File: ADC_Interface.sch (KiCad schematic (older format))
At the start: 18 parts

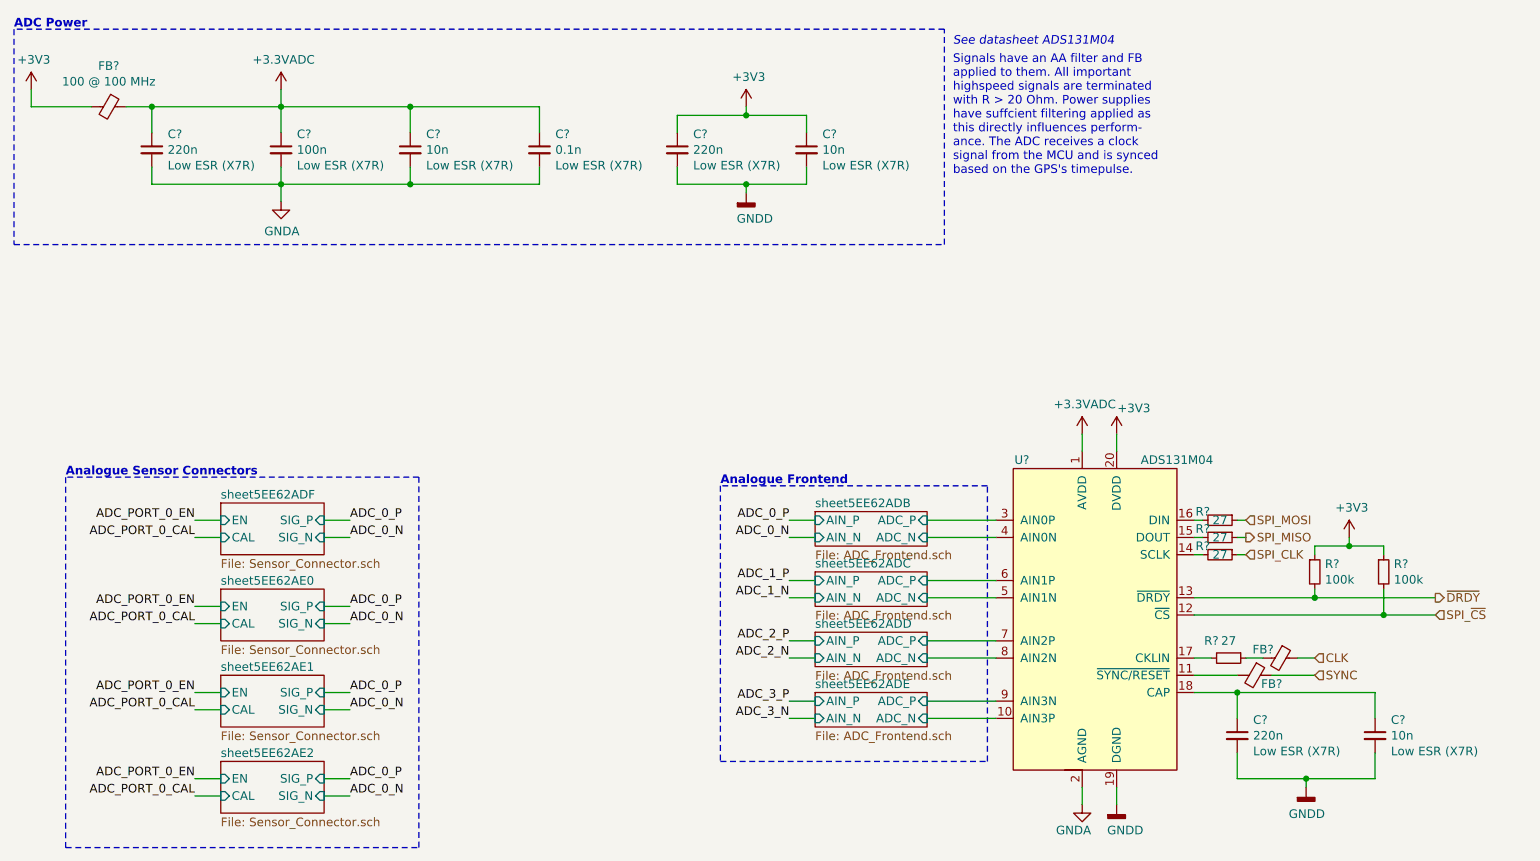
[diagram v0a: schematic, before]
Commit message: Design Mic. Board
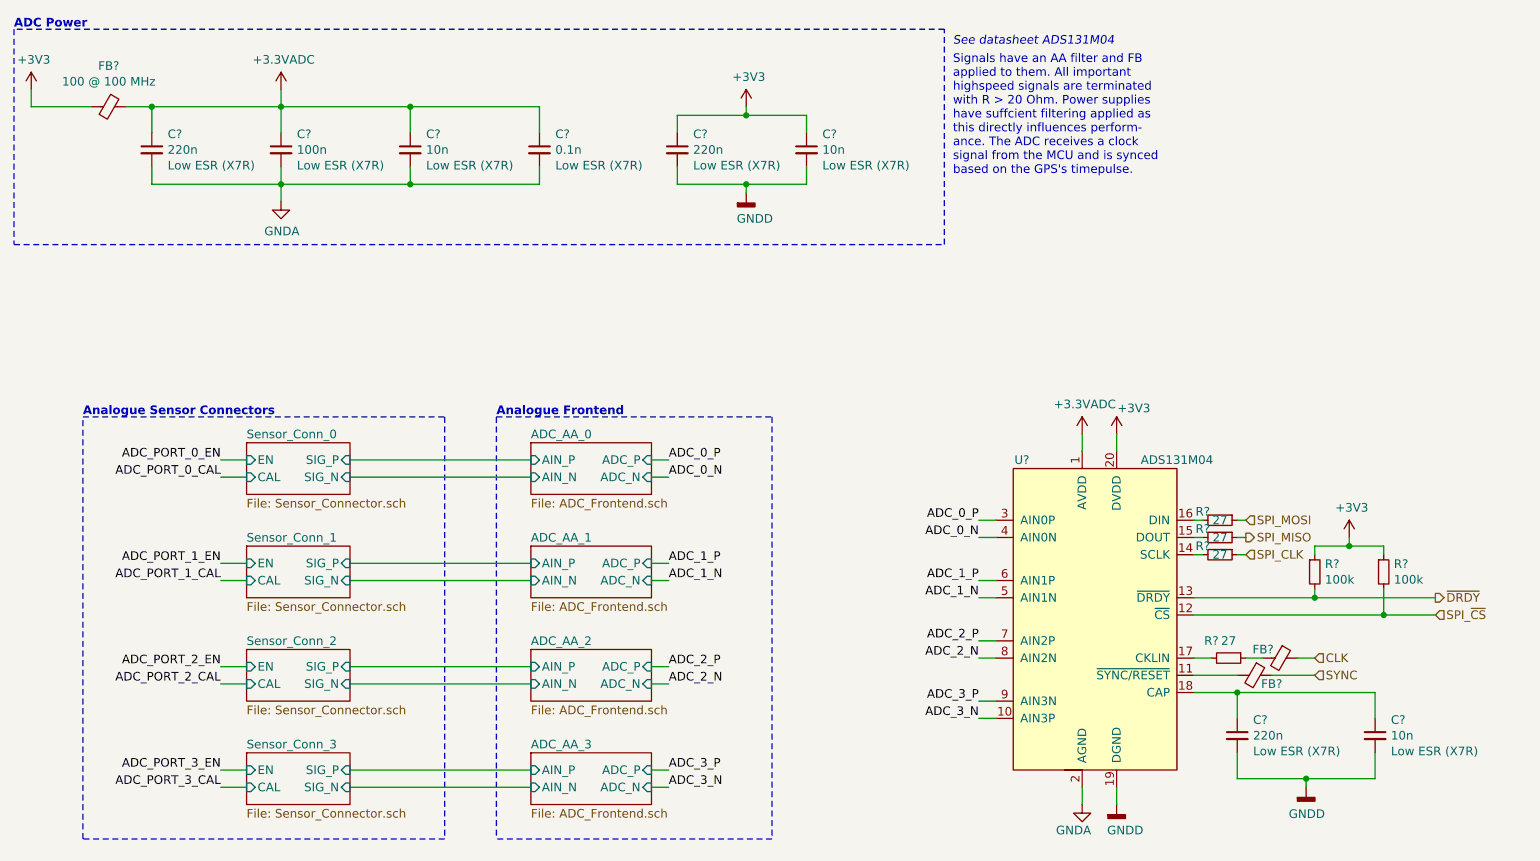
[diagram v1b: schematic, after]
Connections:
- net sheet5EE62ADB/ADC_N is gone; now on net ADC_0_N: U?.4 (AIN0N)
- net sheet5EE62ADB/ADC_P is gone; now on net ADC_0_P: U?.3 (AIN0P)
- net sheet5EE62ADC/ADC_N is gone; now on net ADC_1_N: U?.5 (AIN1N)
- net sheet5EE62ADC/ADC_P is gone; now on net ADC_1_P: U?.6 (AIN1P)
- net sheet5EE62ADD/ADC_N is gone; now on net ADC_2_N: U?.8 (AIN2N)
- net sheet5EE62ADD/ADC_P is gone; now on net ADC_2_P: U?.7 (AIN2P)
- net sheet5EE62ADE/ADC_N is gone; now on net ADC_3_N: U?.10 (AIN3P)
- net sheet5EE62ADE/ADC_P is gone; now on net ADC_3_P: U?.9 (AIN3N)
